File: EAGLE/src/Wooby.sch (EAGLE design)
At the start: 30 parts, among them J1 691210910002, J2 691210910002, J3 691210910002, J4 691210910002, J5 691210910002

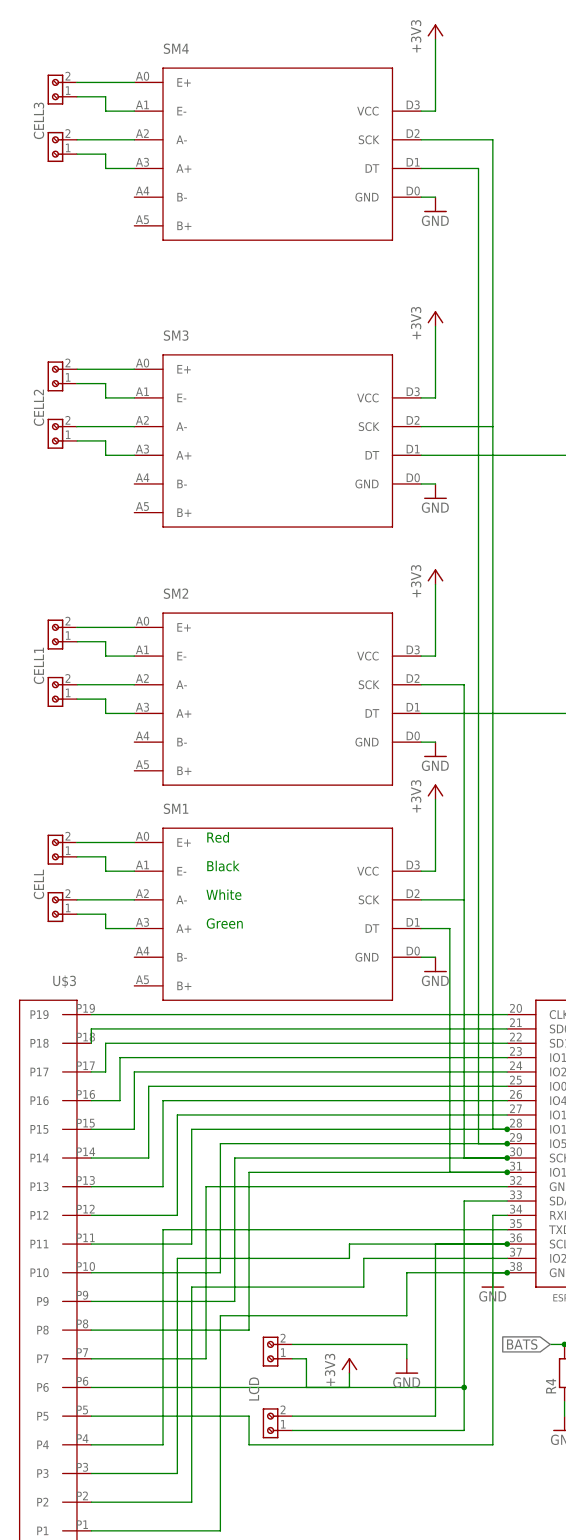
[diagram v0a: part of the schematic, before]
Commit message: Lady D Version
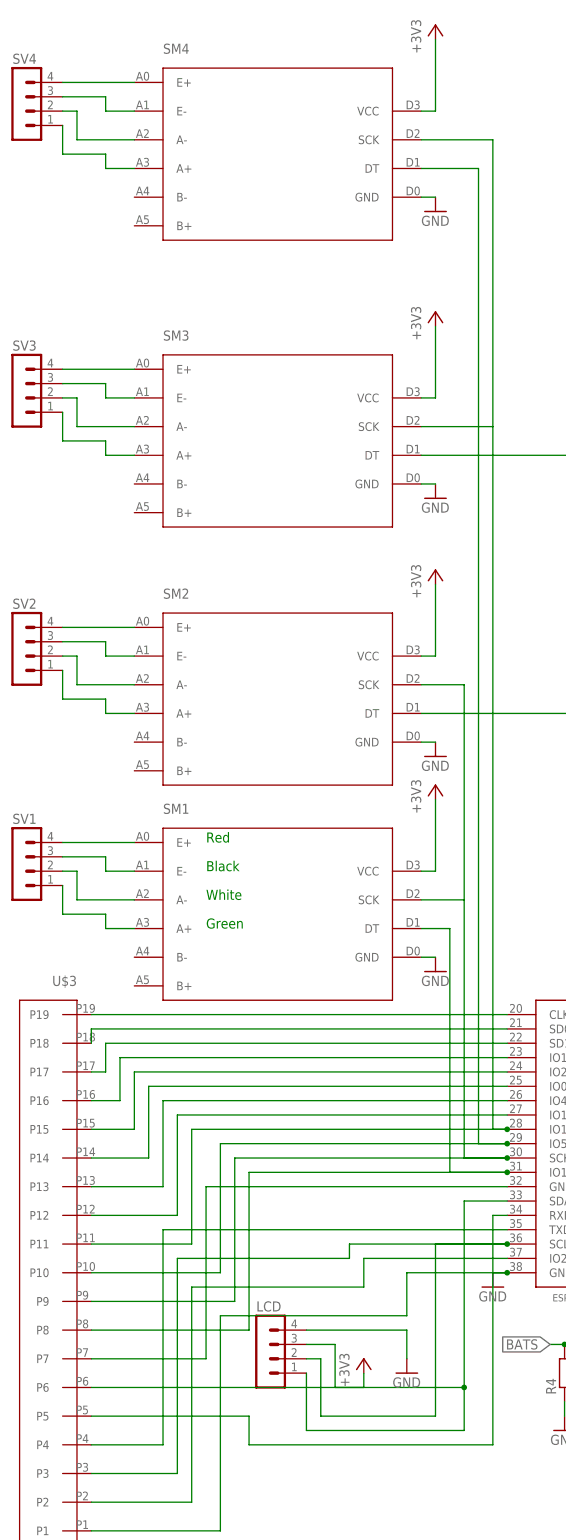
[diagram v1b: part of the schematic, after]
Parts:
- removed CELL, CELL1, CELL2, CELL3, J1, J2, J3, J4, J5: 691210910002, 691210910002:691210910002
- added SV1, SV2, SV3, SV4: (no value), con-lstb:MA04-1
- LCD: value 691210910002 -> (none); device 691210910002:691210910002 -> con-lstb:MA04-1
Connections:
- net +3V3: now also LCD.3; no longer LCD.1
- net GND: now also LCD.4; no longer LCD.2
- net N$1: now also SV1.3; no longer CELL.1
- net N$13: now also SV4.4; no longer CELL3.2
- net N$14: now also SV4.3; no longer CELL3.1
- net N$15: now also SV4.2; no longer J4.2
- net N$16: now also SV4.1; no longer J4.1
- net N$17: now also SV3.4; no longer CELL2.2
- net N$18: now also SV3.3; no longer CELL2.1
- net N$19: now also SV3.2; no longer J3.2
- net N$2: now also SV1.4; no longer CELL.2
- net N$20: now also SV3.1; no longer J3.1
- net N$21: now also SV2.4; no longer CELL1.2
- net N$22: now also SV2.3; no longer CELL1.1
- net N$23: now also SV2.2; no longer J1.2
- net N$24: now also SV2.1; no longer J1.1
- net N$3: now also SV1.1; no longer J5.1
- net N$4: now also SV1.2; no longer J5.2
- net N$6: now also LCD.2; no longer J2.2
- net N$7: now also LCD.1; no longer J2.1
